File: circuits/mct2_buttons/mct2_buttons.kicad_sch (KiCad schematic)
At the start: 35 parts, among them J1 Conn_01x08, SW1 B3F-1052, SW10 B3F-1052, SW11 B3F-1052, SW12 B3F-1052, SW13 OS102011MS2QN1C, SW14 OS102011MS2QN1C, SW2 B3F-1052, SW3 B3F-1052, SW4 B3F-1052, SW5 B3F-1052, SW6 B3F-1052, SW7 B3F-1052, SW8 B3F-1052, SW9 B3F-1052, U1 TCA8418

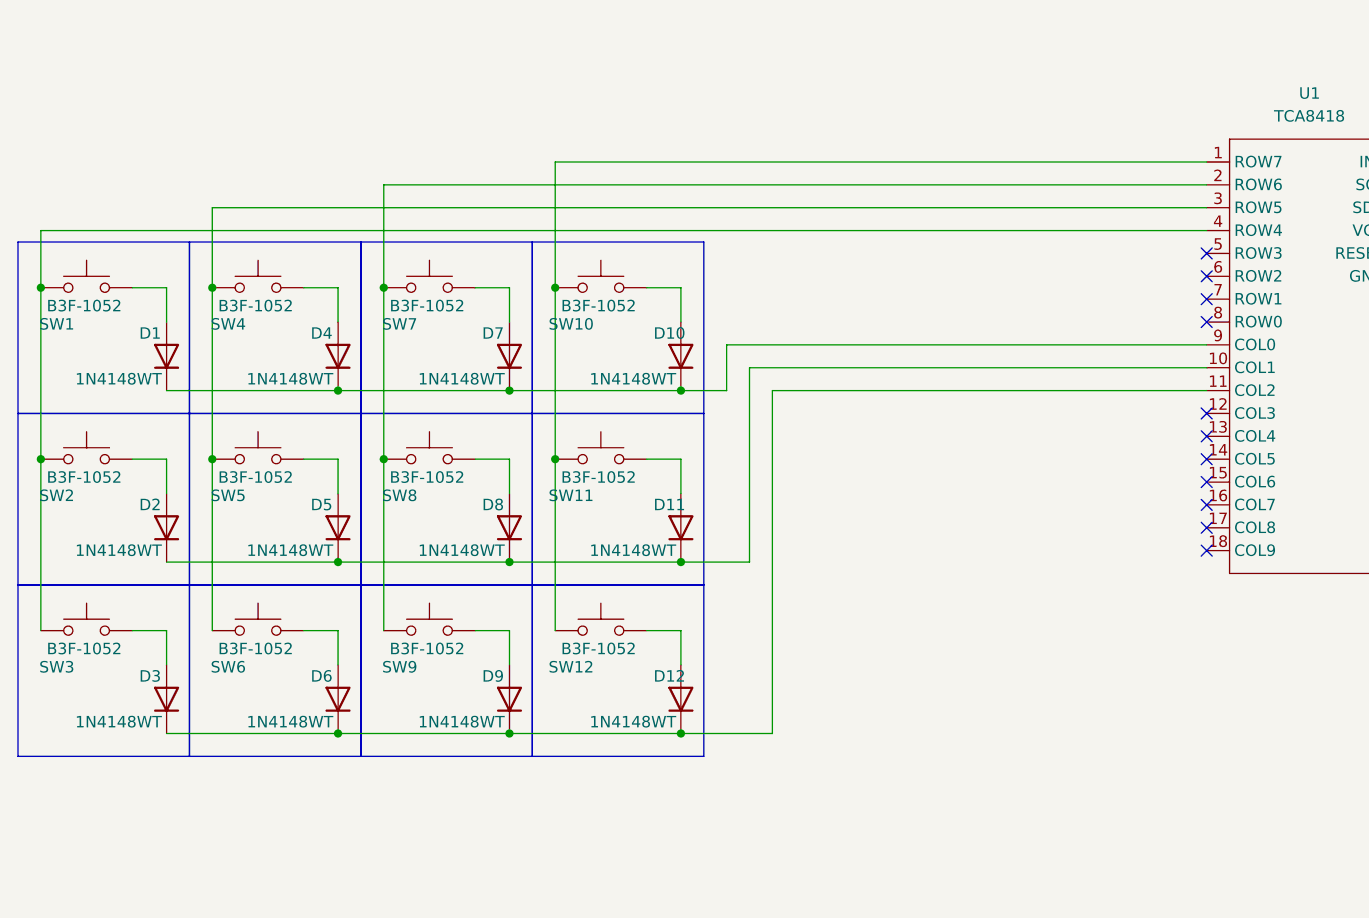
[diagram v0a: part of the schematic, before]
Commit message: Aug 3, 2024
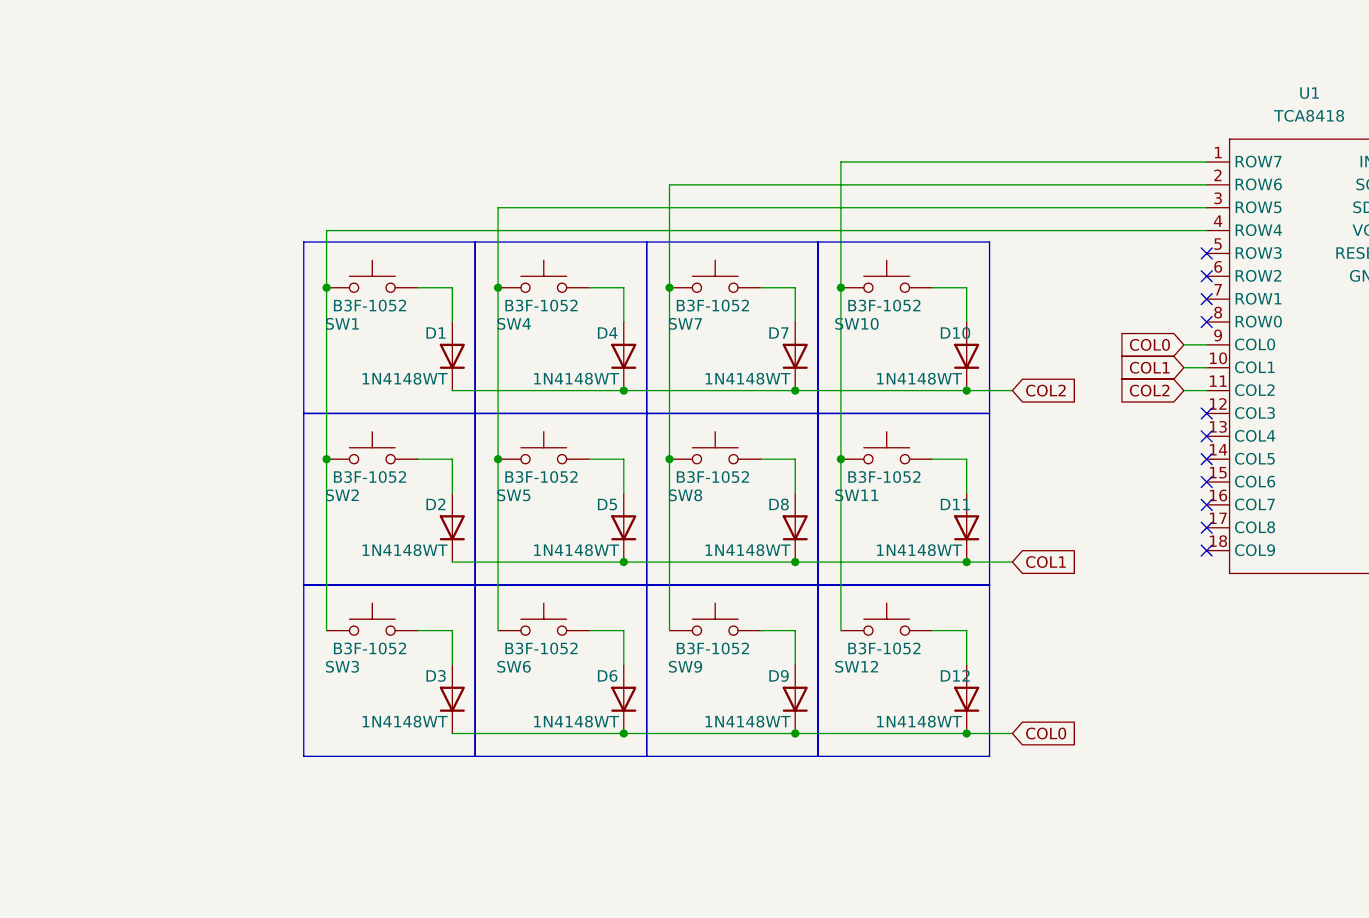
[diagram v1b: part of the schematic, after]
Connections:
- net COL2: now reaches D1.1 (K), D10.1 (K), D4.1 (K), D7.1 (K)
- net COL2: now also U1.11 (COL2); no longer U1.9 (COL0)
- net COL1: now reaches D11.1 (K), D2.1 (K), D5.1 (K), D8.1 (K), U1.10 (COL1)
- net COL0: now reaches D12.1 (K), D3.1 (K), D6.1 (K), D9.1 (K)
- net COL0: now also U1.9 (COL0); no longer U1.11 (COL2)
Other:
- moved on the sheet: D1, D10, D11, D12, D2, D3, D4, D5, D6, D7, D8, D9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
